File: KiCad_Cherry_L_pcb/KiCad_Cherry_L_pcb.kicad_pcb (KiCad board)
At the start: 2 copper layers, 135.7 x 97.6 mm, 0 parts

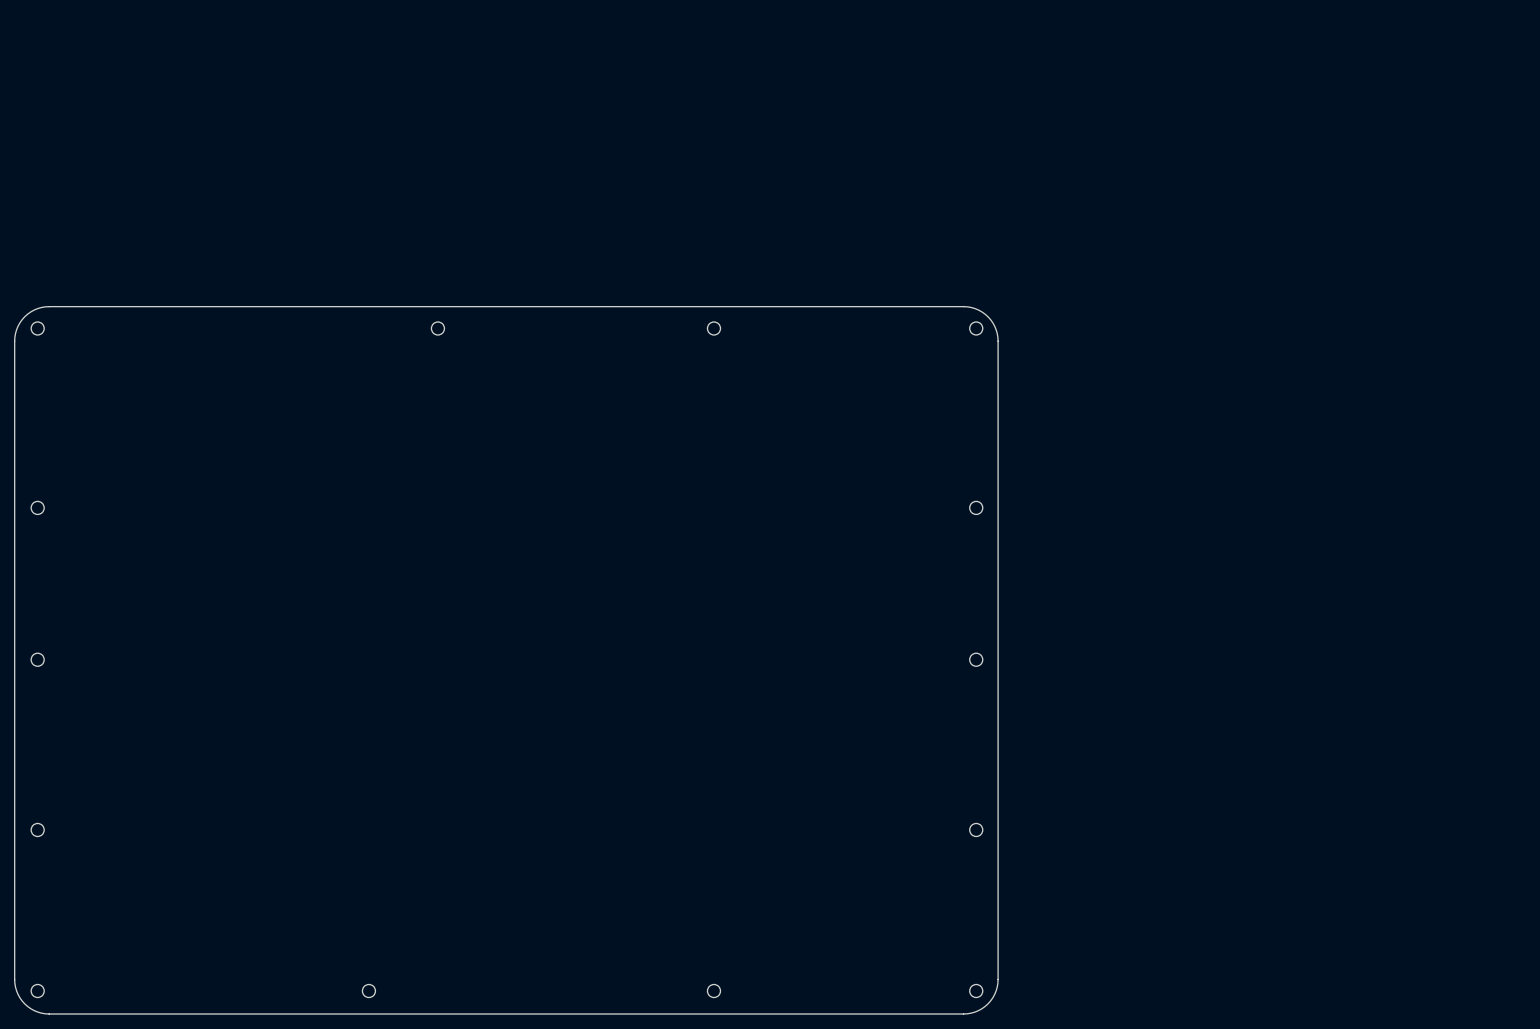
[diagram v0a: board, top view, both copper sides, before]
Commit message: refactor: 作り直し
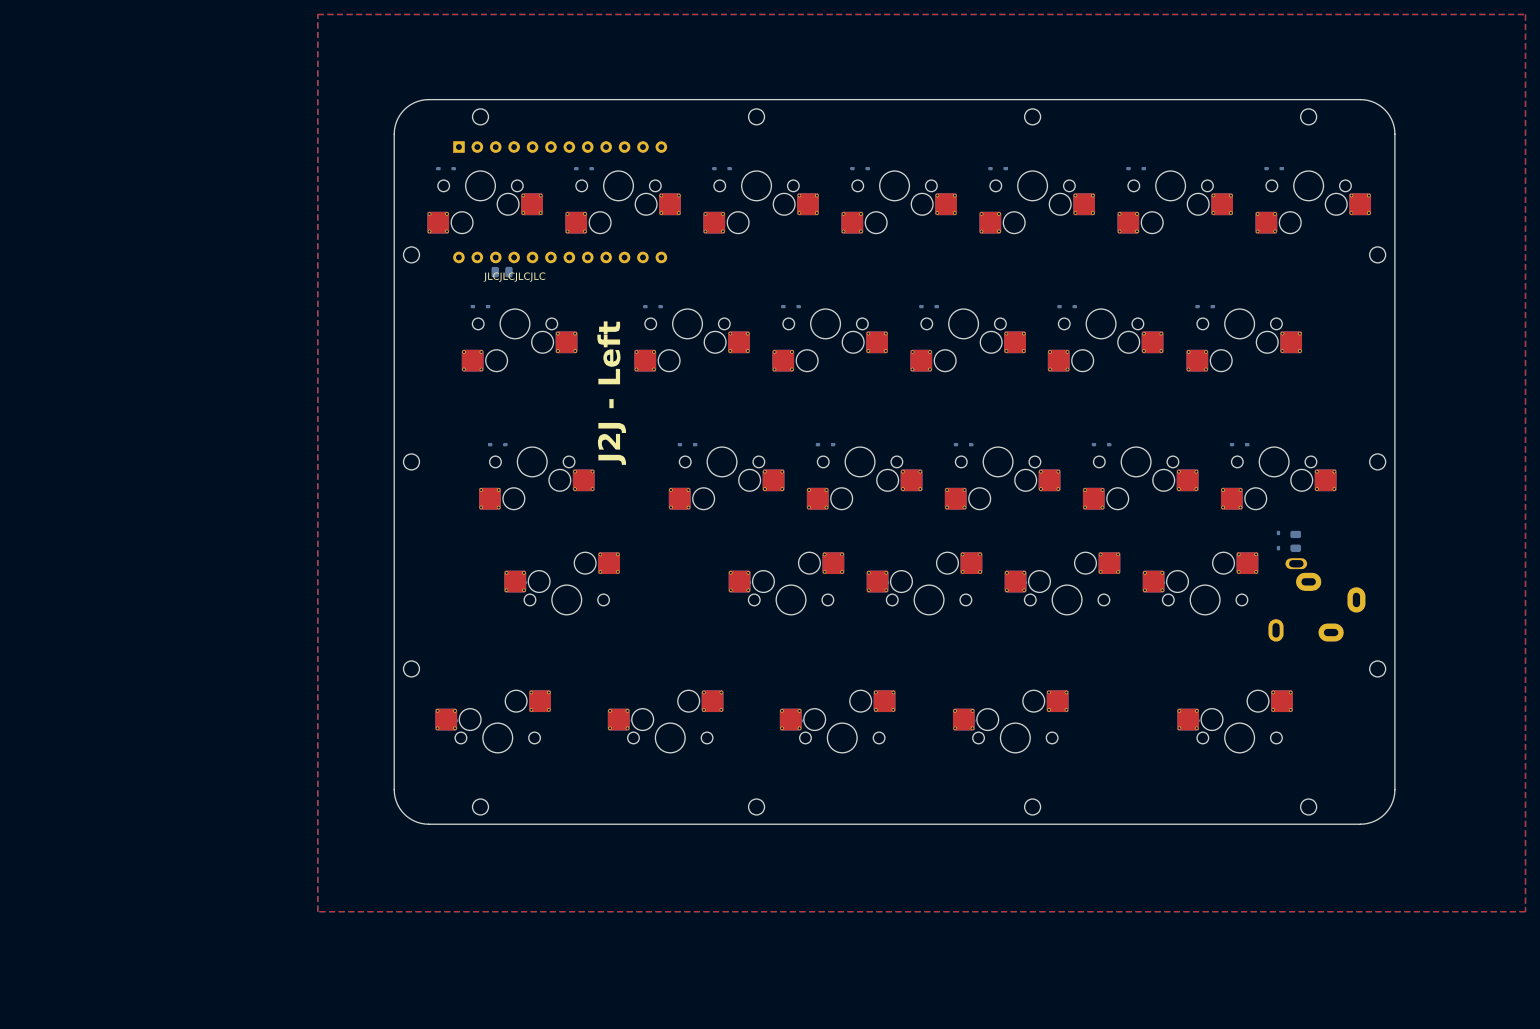
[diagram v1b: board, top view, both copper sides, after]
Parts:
- added C1: C, Capacitor_SMD:C_0805_2012Metric, B.Cu at (205.4, 106.2)
- added C2: C, Capacitor_SMD:C_0805_2012Metric, B.Cu at (95.8, 69.1)
- added D1: 1N4148W, Diode_SMD:D_SOD-323, B.Cu at (88.1, 54.8)
- added D10: 1N4148W, Diode_SMD:D_SOD-323, B.Cu at (154.8, 73.8)
- added D11: 1N4148W, Diode_SMD:D_SOD-323, B.Cu at (173.8, 73.8)
- added D12: 1N4148W, Diode_SMD:D_SOD-323, B.Cu at (192.9, 73.8)
- added D13: 1N4148W, Diode_SMD:D_SOD-323, B.Cu at (95.2, 92.9)
- added D14: 1N4148W, Diode_SMD:D_SOD-323, B.Cu at (121.4, 92.9)
- added D15: 1N4148W, Diode_SMD:D_SOD-323, B.Cu at (140.5, 92.9)
- added D16: 1N4148W, Diode_SMD:D_SOD-323, B.Cu at (159.5, 92.9)
- added D17: 1N4148W, Diode_SMD:D_SOD-323, B.Cu at (178.6, 92.9)
- added D18: 1N4148W, Diode_SMD:D_SOD-323, B.Cu at (197.6, 92.9)
- added D19: 1N4148W, Diode_SMD:D_SOD-323, B.Cu at (100.0, 111.9)
- added D2: 1N4148W, Diode_SMD:D_SOD-323, B.Cu at (107.2, 54.8)
- added D20: 1N4148W, Diode_SMD:D_SOD-323, B.Cu at (131.0, 111.9)
- added D21: 1N4148W, Diode_SMD:D_SOD-323, B.Cu at (150.0, 111.9)
- added D22: 1N4148W, Diode_SMD:D_SOD-323, B.Cu at (169.1, 111.9)
- added D23: 1N4148W, Diode_SMD:D_SOD-323, B.Cu at (188.1, 111.9)
- added D24: 1N4148W, Diode_SMD:D_SOD-323, B.Cu at (202.4, 54.8)
- added D25: 1N4148W, Diode_SMD:D_SOD-323, B.Cu at (90.5, 131.0)
- added D26: 1N4148W, Diode_SMD:D_SOD-323, B.Cu at (114.3, 131.0)
- added D27: 1N4148W, Diode_SMD:D_SOD-323, B.Cu at (138.1, 131.0)
- added D28: 1N4148W, Diode_SMD:D_SOD-323, B.Cu at (161.9, 131.0)
- added D29: 1N4148W, Diode_SMD:D_SOD-323, B.Cu at (192.9, 131.0)
- added D3: 1N4148W, Diode_SMD:D_SOD-323, B.Cu at (126.2, 54.8)
- added D30: 1N4148W, Diode_SMD:D_SOD-323, B.Cu at (203.0, 106.1)
- added D4: 1N4148W, Diode_SMD:D_SOD-323, B.Cu at (145.3, 54.8)
- added D5: 1N4148W, Diode_SMD:D_SOD-323, B.Cu at (164.3, 54.8)
- added D6: 1N4148W, Diode_SMD:D_SOD-323, B.Cu at (183.4, 54.8)
- added D7: 1N4148W, Diode_SMD:D_SOD-323, B.Cu at (92.9, 73.8)
- added D8: 1N4148W, Diode_SMD:D_SOD-323, B.Cu at (116.7, 73.8)
- added D9: 1N4148W, Diode_SMD:D_SOD-323, B.Cu at (135.7, 73.8)
- added H10: MountingHole_2.2mm_M2, MountingHole:MountingHole_2.2mm_M2, F.Cu at (207.2, 47.6)
- added H12: MountingHole_2.2mm_M2, MountingHole:MountingHole_2.2mm_M2, F.Cu at (169.1, 142.9)
- added H13: MountingHole_2.2mm_M2, MountingHole:MountingHole_2.2mm_M2, F.Cu at (207.2, 142.9)
- added H14: MountingHole_2.2mm_M2, MountingHole:MountingHole_2.2mm_M2, F.Cu at (216.7, 123.8)
- added H2: MountingHole_2.2mm_M2, MountingHole:MountingHole_2.2mm_M2, F.Cu at (92.9, 47.6)
- added H2: MountingHole_2.2mm_M2, MountingHole:MountingHole_2.2mm_M2, F.Cu at (92.9, 142.9)
- added H2: MountingHole_2.2mm_M2, MountingHole:MountingHole_2.2mm_M2, F.Cu at (131.0, 142.9)
- added H2: MountingHole_2.2mm_M2, MountingHole:MountingHole_2.2mm_M2, F.Cu at (216.7, 95.2)
- added H2: MountingHole_2.2mm_M2, MountingHole:MountingHole_2.2mm_M2, F.Cu at (83.3, 95.2)
- added H3: MountingHole_2.2mm_M2, MountingHole:MountingHole_2.2mm_M2, F.Cu at (131.0, 47.6)
- added H4: MountingHole_2.2mm_M2, MountingHole:MountingHole_2.2mm_M2, F.Cu at (169.1, 47.6)
- added H7: MountingHole_2.2mm_M2, MountingHole:MountingHole_2.2mm_M2, F.Cu at (83.3, 66.7)
- added H8: MountingHole_2.2mm_M2, MountingHole:MountingHole_2.2mm_M2, F.Cu at (216.7, 66.7)
- added H9: MountingHole_2.2mm_M2, MountingHole:MountingHole_2.2mm_M2, F.Cu at (83.3, 123.8)
- added J1: AudioJack3_SwitchTR, Connector_Audio:Jack_3.5mm_CUI_SJ1-3515N_Horizontal, B.Cu at (213.8, 114.3)
- added SW1: Esc, KBD_BrownSugar:CherryMX_Hotswap_via_1U, F.Cu at (92.9, 57.1)
- added SW10: E, KBD_BrownSugar:CherryMX_Hotswap_via_1U, F.Cu at (159.5, 76.2)
- added SW11: R, KBD_BrownSugar:CherryMX_Hotswap_via_1U, F.Cu at (178.5, 76.2)
- added SW12: T, KBD_BrownSugar:CherryMX_Hotswap_via_1U, F.Cu at (197.6, 76.2)
- added SW13: Ctrl, KBD_BrownSugar:CherryMX_Hotswap_via_1.75U, F.Cu at (100.0, 95.2)
- added SW14: A, KBD_BrownSugar:CherryMX_Hotswap_via_1U, F.Cu at (126.2, 95.2)
- added SW15: S, KBD_BrownSugar:CherryMX_Hotswap_via_1U, F.Cu at (145.3, 95.2)
- added SW16: D, KBD_BrownSugar:CherryMX_Hotswap_via_1U, F.Cu at (164.3, 95.2)
- added SW17: F, KBD_BrownSugar:CherryMX_Hotswap_via_1U, F.Cu at (183.4, 95.2)
- added SW18: G, KBD_BrownSugar:CherryMX_Hotswap_via_1U, F.Cu at (202.4, 95.2)
- added SW19: Shift, KBD_BrownSugar:CherryMX_Hotswap_via_2.25U, F.Cu at (104.8, 114.3)
- added SW2: 1, KBD_BrownSugar:CherryMX_Hotswap_via_1U, F.Cu at (111.9, 57.1)
- added SW20: Z, KBD_BrownSugar:CherryMX_Hotswap_via_1U, F.Cu at (135.7, 114.3)
- added SW21: X, KBD_BrownSugar:CherryMX_Hotswap_via_1U, F.Cu at (154.8, 114.3)
- added SW22: C, KBD_BrownSugar:CherryMX_Hotswap_via_1U, F.Cu at (173.8, 114.3)
- added SW23: V, KBD_BrownSugar:CherryMX_Hotswap_via_1U, F.Cu at (192.9, 114.3)
- added SW24: 6, KBD_BrownSugar:CherryMX_Hotswap_via_1U, F.Cu at (207.2, 57.1)
- added SW25: Fn, KBD_BrownSugar:CherryMX_Hotswap_via_1.25U, F.Cu at (95.3, 133.3)
- added SW26: Alt, KBD_BrownSugar:CherryMX_Hotswap_via_1.25U, F.Cu at (119.1, 133.3)
- added SW27: Win, KBD_BrownSugar:CherryMX_Hotswap_via_1.25U, F.Cu at (142.8, 133.3)
- added SW28: NoConv, KBD_BrownSugar:CherryMX_Hotswap_via_1.25U, F.Cu at (166.7, 133.3)
- added SW29: Space, KBD_BrownSugar:CherryMX_Hotswap_via_2U, F.Cu at (197.6, 133.3)
- added SW3: 2, KBD_BrownSugar:CherryMX_Hotswap_via_1U, F.Cu at (131.0, 57.1)
- added SW4: 3, KBD_BrownSugar:CherryMX_Hotswap_via_1U, F.Cu at (150.0, 57.1)
- added SW5: 4, KBD_BrownSugar:CherryMX_Hotswap_via_1U, F.Cu at (169.1, 57.1)
- added SW6: 5, KBD_BrownSugar:CherryMX_Hotswap_via_1U, F.Cu at (188.1, 57.1)
- added SW7: Tab, KBD_BrownSugar:CherryMX_Hotswap_via_1.5U, F.Cu at (97.6, 76.2)
- added SW8: Q, KBD_BrownSugar:CherryMX_Hotswap_via_1U, F.Cu at (121.4, 76.2)
- added SW9: W, KBD_BrownSugar:CherryMX_Hotswap_via_1U, F.Cu at (140.5, 76.2)
- added U1: Sparkfun_Pro_Micro, Arduino:Sparkfun_Pro_Micro, B.Cu at (117.8, 67.0)
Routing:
- added copper zone on B.Cu, net GND
- added copper zone on F.Cu, net GND
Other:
- board size 135.7 x 97.6 mm -> 138.1 x 100 mm
- board text added: "J2J - Left"
- board text added: "JLCJLCJLCJLC"

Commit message: feat: Rightの配置が完了
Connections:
- U1 pad 12: +5V -> unconnected-(U1-~D9/A9-Pad12)
- U1 pad 13: unconnected-(U1-~D10/A10-Pad13) -> +5V
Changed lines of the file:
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@@
 	(net 39 "unconnected-(J1-PadRN)")
 	(net 40 "SCL")
-	(net 41 "unconnected-(U1-~D10{slash}A10-Pad13)")
+	(net 41 "unconnected-(U1-~D9{slash}A9-Pad12)")
 	(net 42 "Col0")
 	(net 43 "Col1")
@@
 			(layers "*.Cu" "*.Mask")
 			(remove_unused_layers no)
-			(net 1 "+5V")
+			(net 41 "unconnected-(U1-~D9{slash}A9-Pad12)")
 			(pinfunction "~D9/A9")
-			(pintype "bidirectional")
+			(pintype "bidirectional+no_connect")
 		)
 		(pad "13" thru_hole oval
@@
 			(layers "*.Cu" "*.Mask")
 			(remove_unused_layers no)
-			(net 41 "unconnected-(U1-~D10{slash}A10-Pad13)")
+			(net 1 "+5V")
 			(pinfunction "~D10/A10")
-			(pintype "bidirectional+no_connect")
+			(pintype "bidirectional")
 		)
 		(pad "14" thru_hole oval
@@
 			(net 49 "unconnected-(U1-RST-Pad22)")
 			(pinfunction "RST")
-			(pintype "input")
+			(pintype "input+no_connect")
 		)
 		(pad "23" thru_hole oval
